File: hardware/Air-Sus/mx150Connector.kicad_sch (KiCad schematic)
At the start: 25 parts, among them J4 MX150_02x06_Vertical

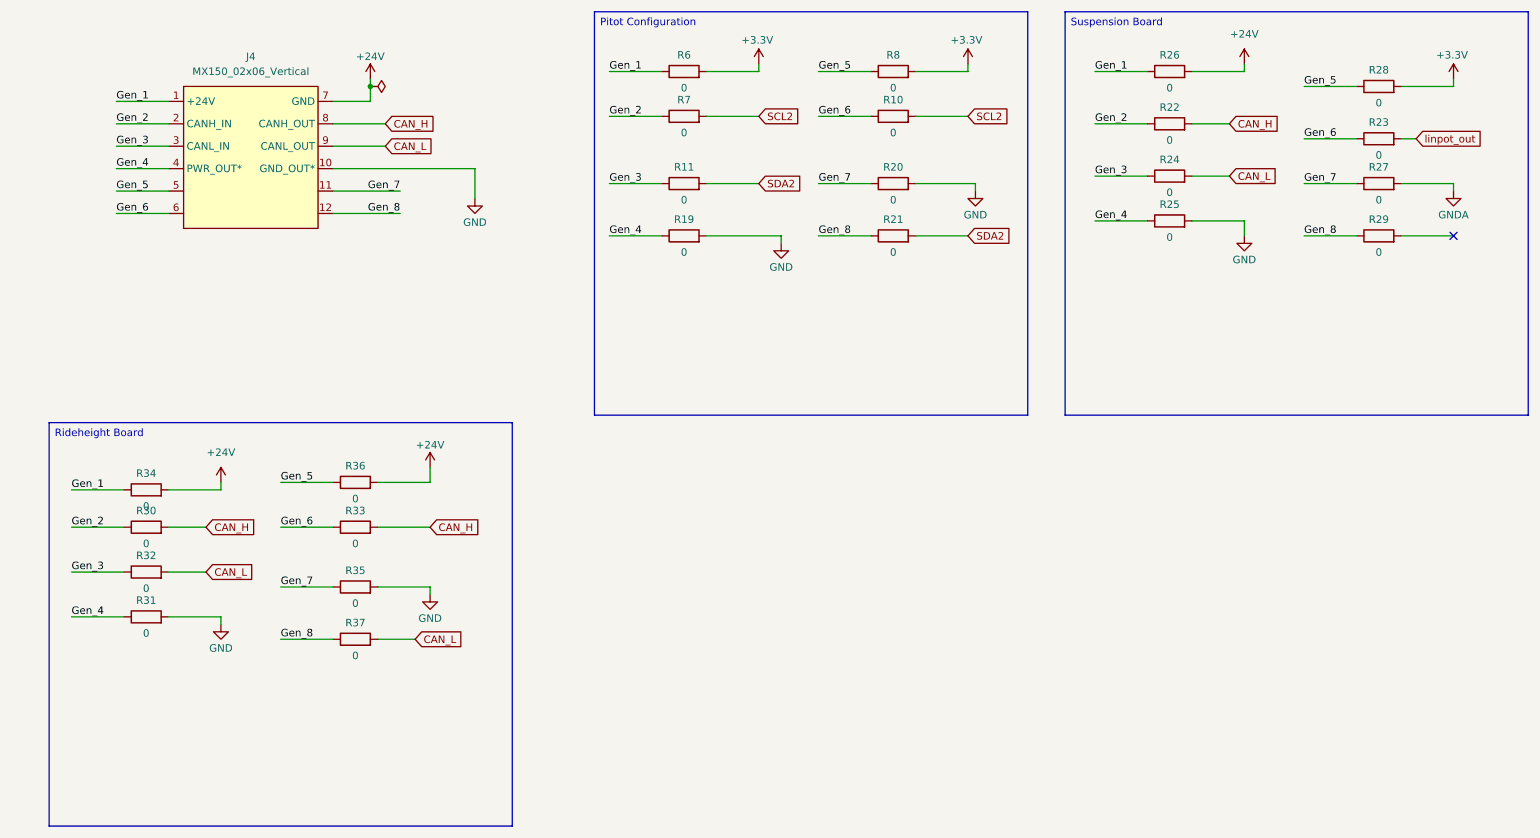
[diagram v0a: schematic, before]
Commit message: air-sus layout check e Please enter the commit message for your changes. Lines starting
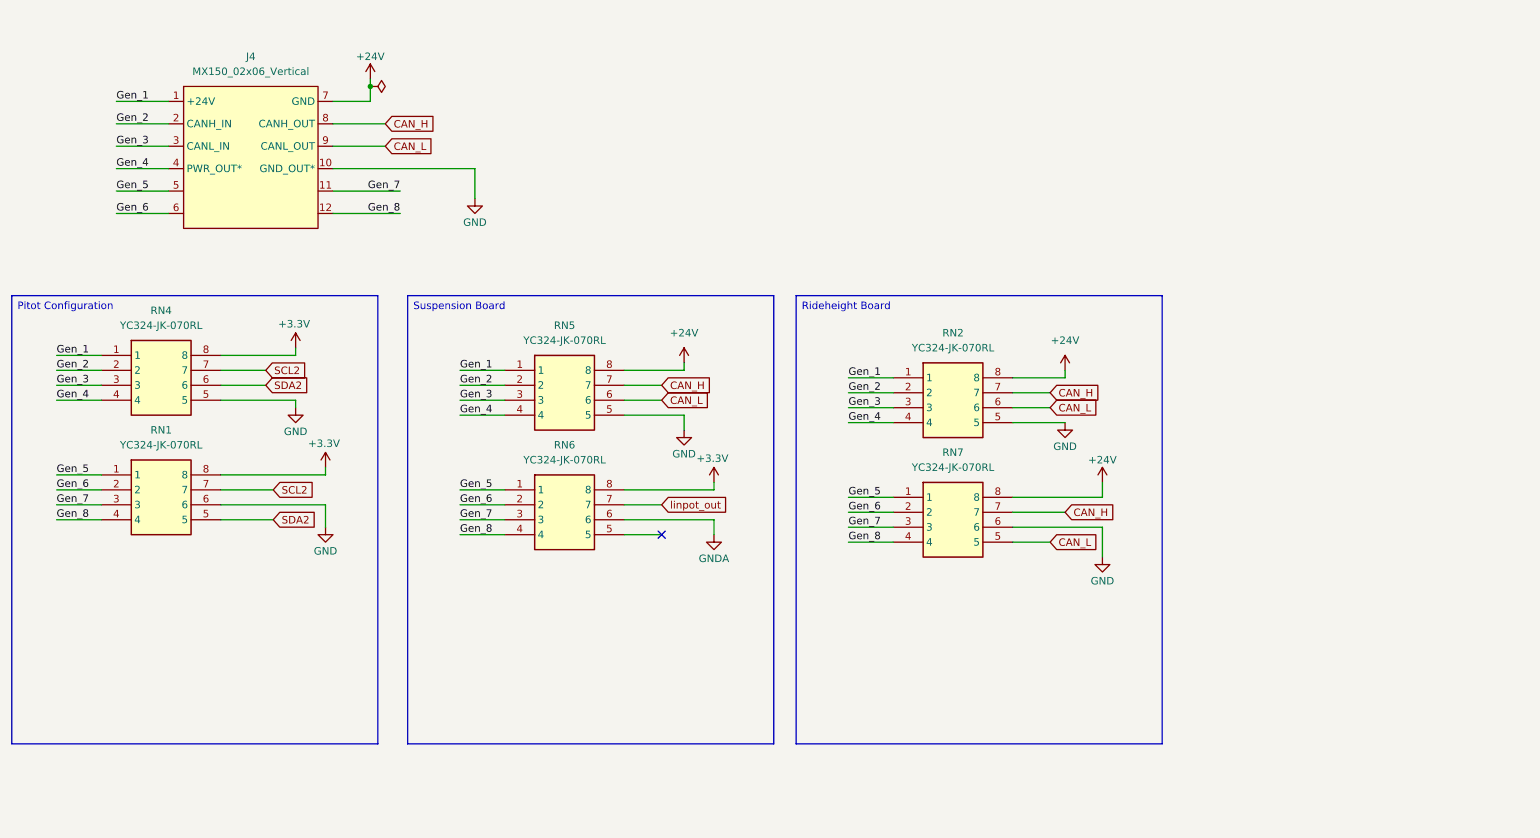
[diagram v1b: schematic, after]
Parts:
- removed R10, R11, R19, R20, R21, R22, R23, R24, R25, R26, R27, R28, R29, R30, R31, R32, R33, R34, R35, R36, R37, R6, R7, R8: 0, Resistor_SMD:R_0603_1608Metric_Pad0.98x0.95mm_HandSolder, symbol Device:R
- added RN1, RN2, RN4, RN5, RN6, RN7: YC324-JK-070RL, 4pinRes:YC324JK07220RL, symbol 4PinConn:YC324-JK-070RL
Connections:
- net +24V: now also RN2.8, RN5.8, RN7.8
- net +3.3V: now also RN1.8, RN4.8, RN6.8
- net CAN_H: now also RN2.7, RN5.7, RN7.7
- net CAN_L: now also RN2.6, RN5.6, RN7.5
- net GND: now also RN1.6, RN2.5, RN4.5, RN5.5, RN7.6
- net GNDA: now also RN6.6
- net Gen_1: now also RN2.1, RN4.1, RN5.1
- net Gen_2: now also RN2.2, RN4.2, RN5.2
- net Gen_3: now also RN2.3, RN4.3, RN5.3
- net Gen_4: now also RN2.4, RN4.4, RN5.4
- net Gen_5: now also RN1.1, RN6.1, RN7.1
- net Gen_6: now also RN1.2, RN6.2, RN7.2
- net Gen_7: now also RN1.3, RN6.3, RN7.3
- net Gen_8: now also RN1.4, RN6.4, RN7.4
- net SCL2: now also RN1.7, RN4.7
- net SDA2: now also RN1.5, RN4.6
- net linpot_out: now also RN6.7
